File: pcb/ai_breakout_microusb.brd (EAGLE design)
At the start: 10.2 x 14.2 mm, 4 parts, among them J1 1X04NFNS, J2 1X04NFNS

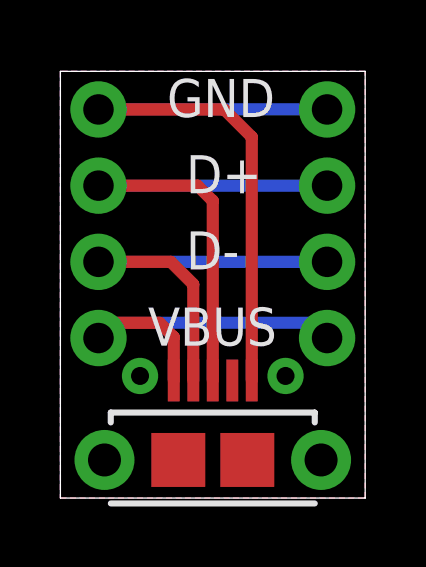
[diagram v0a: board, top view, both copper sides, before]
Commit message: ready for manufacturing
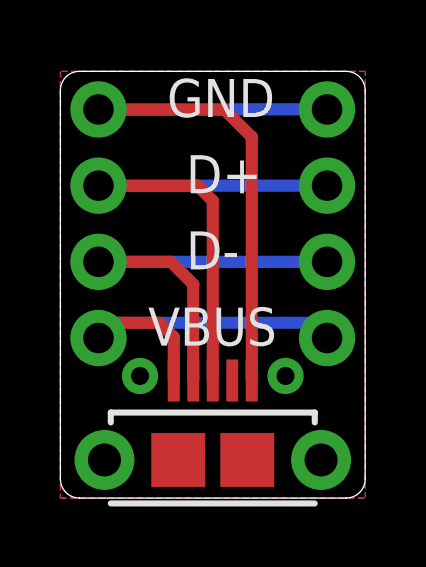
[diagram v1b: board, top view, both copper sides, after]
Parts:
- removed U$1: (no value), Ai_Miscellany:AI-LOGO-XS
- added U$2: AI-LOGOXS, Ai_Miscellany:AI-LOGO-XS
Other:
- outline, holes or cut-outs redrawn
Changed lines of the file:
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@@
 <board>
 <plain>
-<wire x1="10.16" y1="0" x2="10.16" y2="14.224" width="0.0254" layer="20"/>
-<wire x1="10.16" y1="14.224" x2="0" y2="14.224" width="0.0254" layer="20"/>
-<wire x1="0" y1="14.224" x2="0" y2="0" width="0.0254" layer="20"/>
-<wire x1="0" y1="0" x2="10.16" y2="0" width="0.0254" layer="20"/>
+<wire x1="0.635" y1="0" x2="9.525" y2="0" width="0.0254" layer="20"/>
+<wire x1="9.525" y1="0" x2="10.16" y2="0.635" width="0.0254" layer="20" curve="90"/>
+<wire x1="10.16" y1="0.635" x2="10.16" y2="13.589" width="0.0254" layer="20"/>
+<wire x1="10.16" y1="13.589" x2="9.525" y2="14.224" width="0.0254" layer="20" curve="90"/>
+<wire x1="9.525" y1="14.224" x2="0.635" y2="14.224" width="0.0254" layer="20"/>
+<wire x1="0.635" y1="14.224" x2="0" y2="13.589" width="0.0254" layer="20" curve="90"/>
+<wire x1="0" y1="13.589" x2="0" y2="0.635" width="0.0254" layer="20"/>
+<wire x1="0" y1="0.635" x2="0.635" y2="0" width="0.0254" layer="20" curve="90"/>
 <text x="6.731" y="12.7" size="1.27" layer="26" font="vector" ratio="10" rot="MR0">GND</text>
 <text x="6.223" y="10.16" size="1.27" layer="26" font="vector" ratio="10" rot="MR0">D+</text>
@@
 </autorouter>
 <elements>
-<element name="U$1" library="Ai_Miscellany" package="AI-LOGO-XS" value="" x="6.477" y="0.889" rot="MR0"/>
 <element name="J1" library="Ai_Connectors" package="1X04-NFNS" value="1X04NFNS" x="1.27" y="9.144" smashed="yes" rot="R90"/>
 <element name="J2" library="Ai_Connectors" package="1X04-NFNS" value="1X04NFNS" x="8.89" y="9.144" smashed="yes" rot="R90"/>
 <element name="USB1" library="Ai_Connectors" package="USB-MICROB-TH" value="USBMICROB-TH" x="5.08" y="1.27"/>
+<element name="U$2" library="Ai_Miscellany" package="AI-LOGO-XS" value="AI-LOGOXS" x="6.477" y="0.635" rot="MR0"/>
 </elements>
 <signals>
